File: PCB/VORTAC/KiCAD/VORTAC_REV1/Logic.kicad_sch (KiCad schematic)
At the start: 26 parts, among them Q3 BSS138AKDW, U1 TLV73333PDBV, U3 EE-SX4320, U5 AS5047D, U6 AP63205WU, U7 EE-SX3350

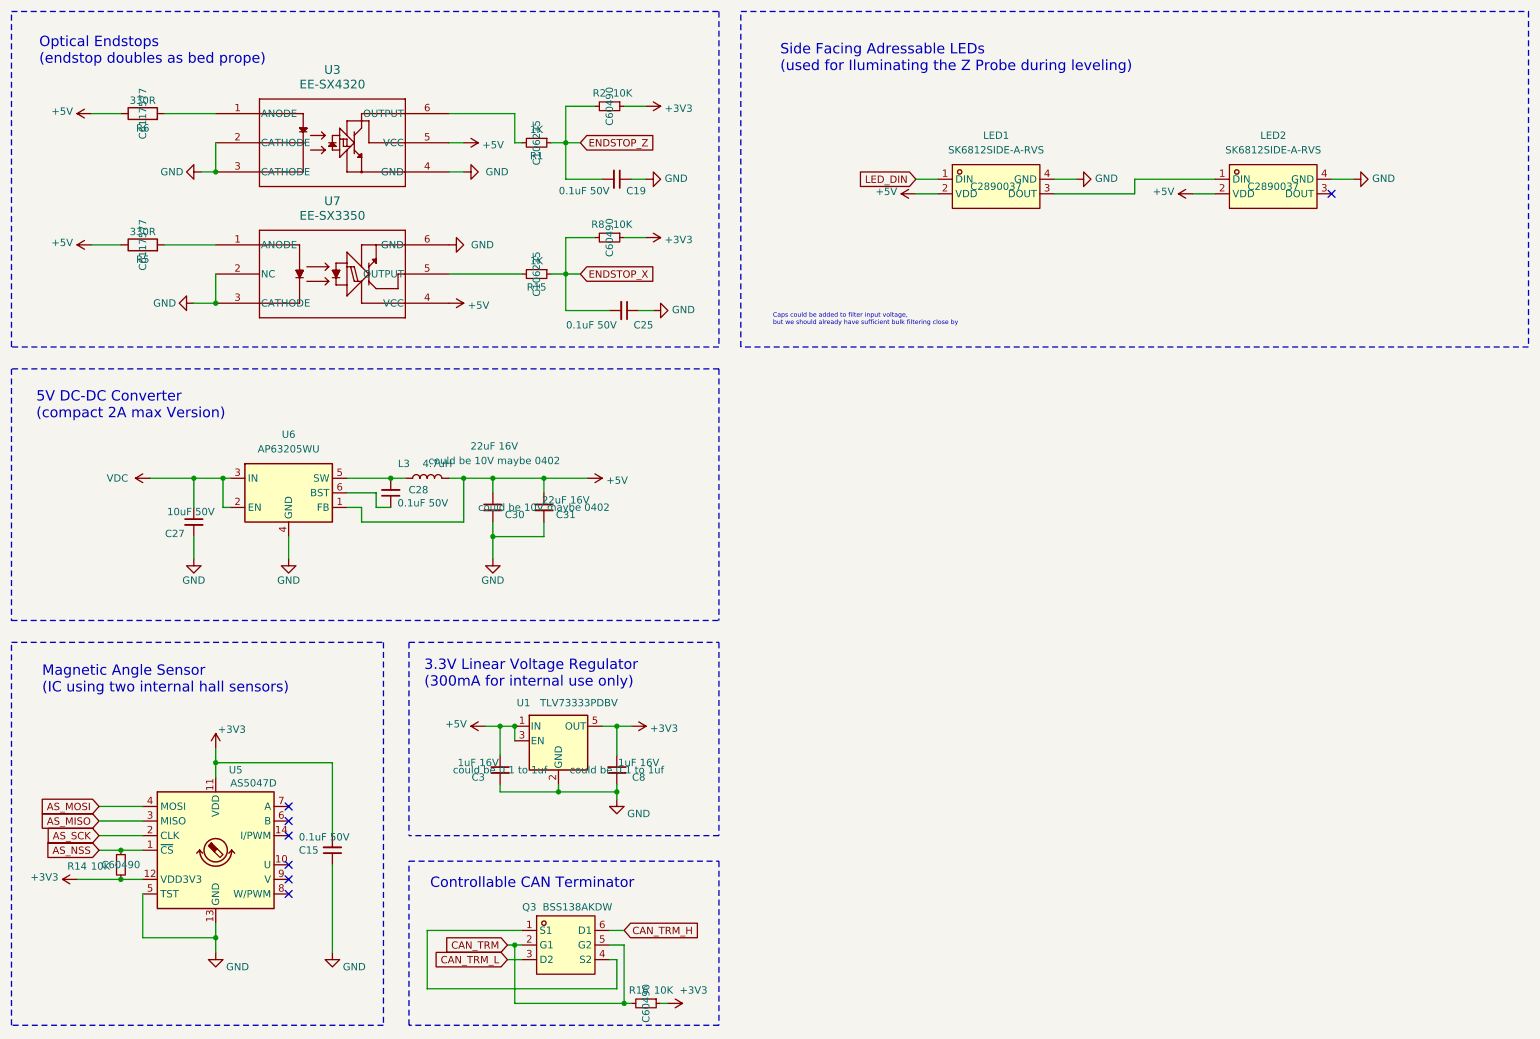
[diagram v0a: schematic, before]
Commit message: Evil Mita is v00:98
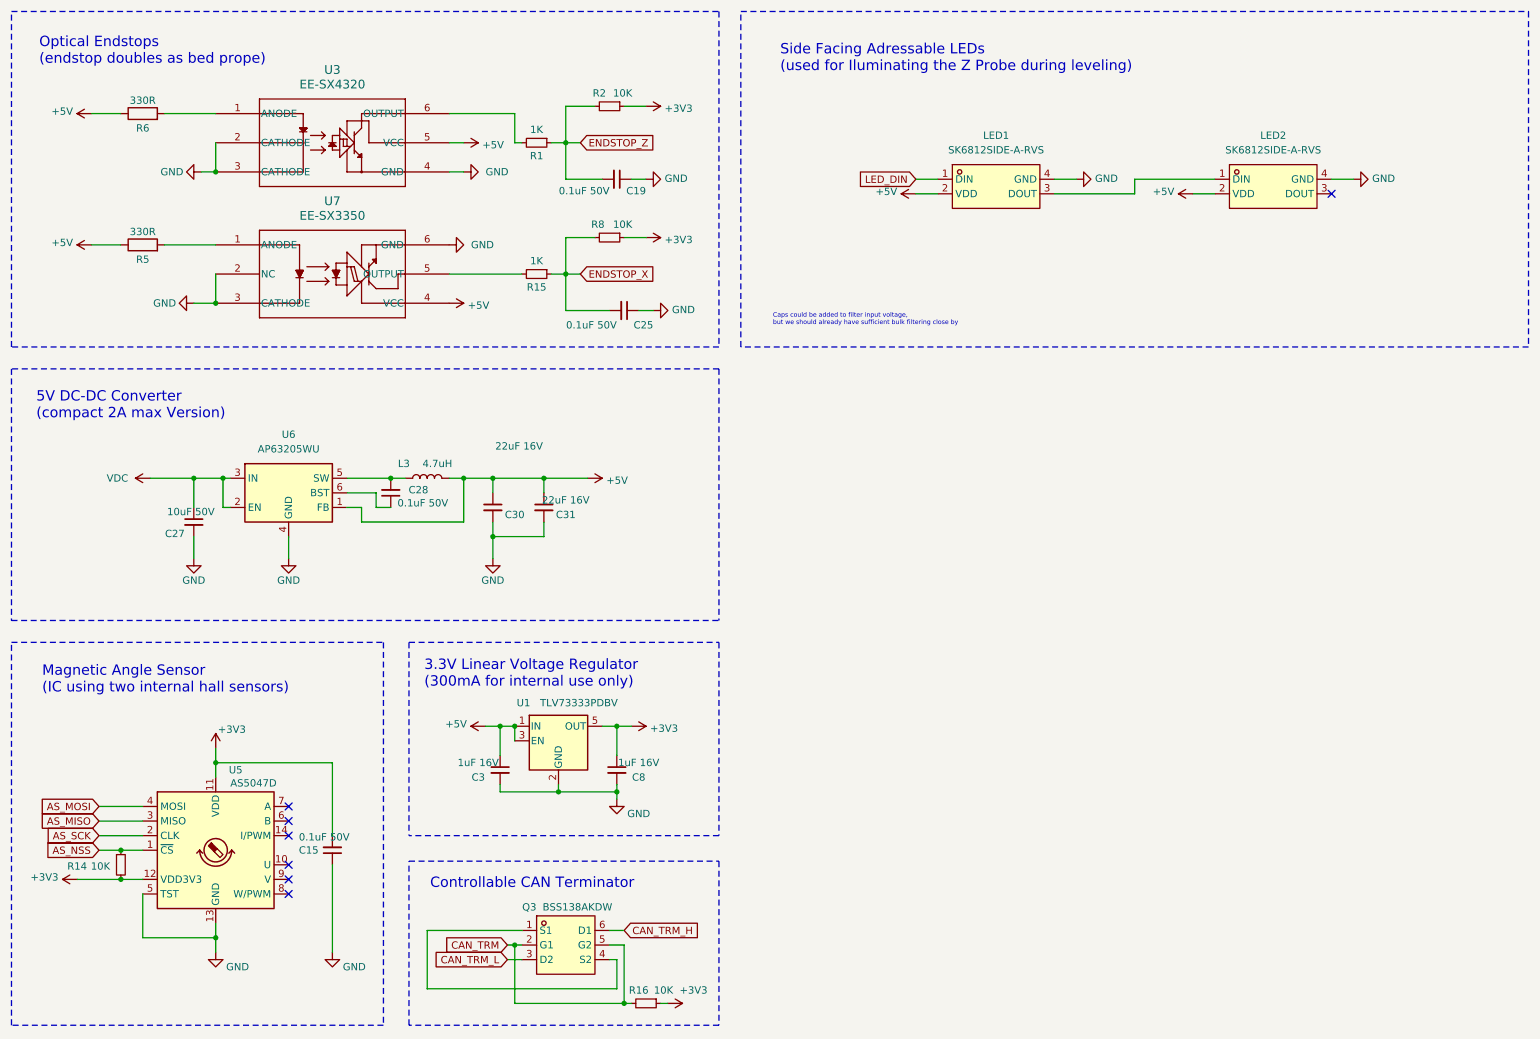
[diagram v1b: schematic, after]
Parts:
- C3, C8: description could be 0.1 to 1uf -> (none); notes (none) -> could be 0.1 to 1uf
- C30, C31: description could be 10V maybe 0402 -> (none); notes (none) -> could be 10V maybe 0402
